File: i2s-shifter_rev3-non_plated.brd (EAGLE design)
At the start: 53 x 47 mm, 31 parts, among them IC1 74HC164D, IC2 74HC164D, IC3 74HC164D, IC4 74HC164D, IC5 74HC164D

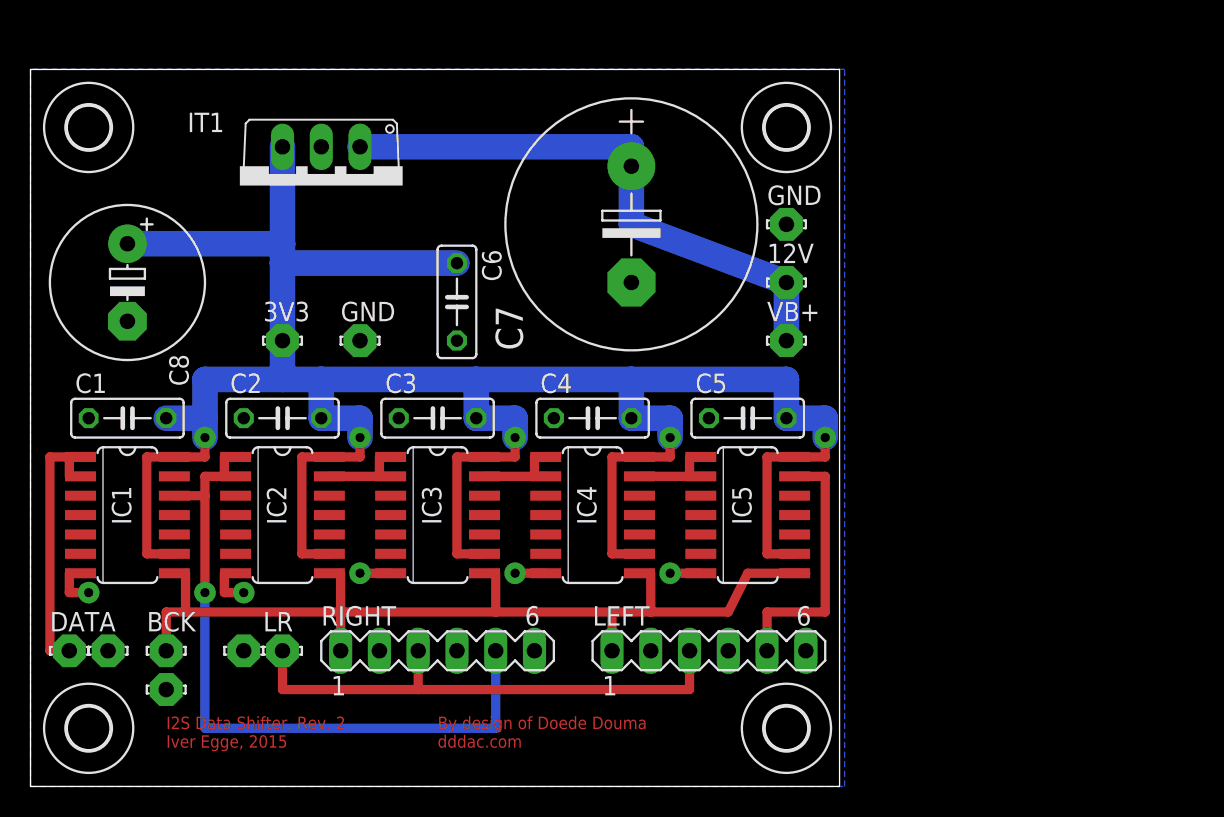
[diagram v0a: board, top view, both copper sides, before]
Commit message: rev3
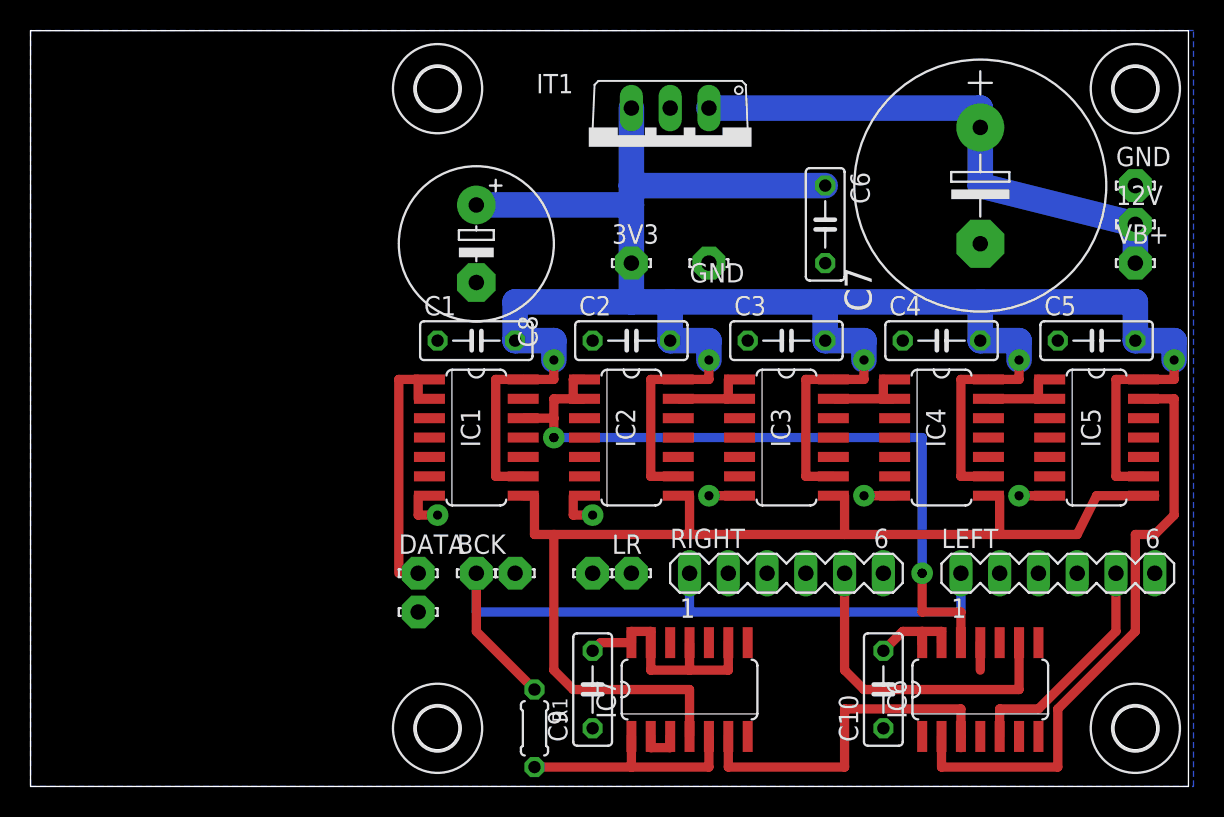
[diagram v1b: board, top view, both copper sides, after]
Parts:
- added C10, C9: (no value), resistor:C050-025X075
- added IC6: 74HC74D, 74xx-eu:SO14
- added IC7: 74HC04D, 74xx-eu:SO14
- added R1: (no value), resistor:0204/5
- moved C6 24.7 mm to (52.1, 36.8)
- moved GND16 24.1 mm to (31.8, 14.0)
- moved GND* 23.4 mm to (44.5, 34.3)
- moved C1 23.4 mm to (29.2, 29.2)
- moved C3 23.4 mm to (49.5, 29.2)
- moved C4 23.4 mm to (59.7, 29.2)
- moved DATA 23.4 mm to (25.4, 14.0)
- moved GND15 23.4 mm to (36.8, 14.0)
- moved IC1 23.4 mm to (29.2, 22.9)
- moved IC3 23.4 mm to (49.5, 22.9)
- moved IC4 23.4 mm to (59.7, 22.9)
- moved LEFT 23.4 mm to (67.3, 14.0)
- moved RIGHT 23.4 mm to (49.5, 14.0)
- moved VB+ 23.4 mm to (72.4, 34.3)
- moved 3V3 23.4 mm to (39.4, 34.3)
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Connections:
- new net +5V: C10.2, C9.2, IC6.1, IC6.10, IC6.13, IC6.14, IC6.4, IC7.11, IC7.13, IC7.14, IC7.9
- new net N$10: BCK.MP, LEFT.1, R1.1, RIGHT.1
- new net N$11: IC7.2, IC7.3
- new net N$12: IC6.11, IC6.3, IC7.6
- new net N$13: IC1.12, IC2.1, IC2.2, IC6.12
- new net N$14: IC7.1, IC7.5, R1.2
- new net N$7: IC6.5, LEFT.5
- net GND: now also C10.1, C9.1, IC6.7, IC7.7
- net N$2: now also IC7.4; no longer BCK.MP, LEFT.1, RIGHT.1
- net N$3: now also IC5.13, IC6.2; no longer IC1.12, IC2.1, IC2.2, RIGHT.5
- net N$8: now also IC6.9, RIGHT.5; no longer IC5.13, LEFT.5
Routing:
- net N$13: track 0.00 -> 49.4 mm, vias 0 -> 2
- net N$10: track 0.00 -> 48.6 mm
- net N$9: track 34.3 -> 0.00 mm
- net N$12: track 0.00 -> 25.4 mm
- net +5V: track 0.00 -> 21.8 mm
- net N$14: track 0.00 -> 15.4 mm
- net N$7: track 0.00 -> 15.3 mm
- net N$2: track 64.9 -> 77.4 mm
- net N$3: track 46.7 -> 39.7 mm, vias 1 -> 0
- net N$8: track 17.2 -> 21.4 mm
- net N$11: track 0.00 -> 2.74 mm
- net +12V: track 37.5 -> 35.9 mm
- net N$1: track 18.0 -> 16.7 mm
- net +3V3: track 172.8 -> 174.1 mm
- net GND: vias 10 -> 12
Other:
- board size 53 x 47 mm -> 75.9 x 49.5 mm
- board text removed: "By design of Doede Douma dddac.com"
- board text removed: "I2S Data Shifter, Rev. 2 Iver Egge, 2015"
